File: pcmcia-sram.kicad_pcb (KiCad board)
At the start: 4 copper layers, 9 parts, among them J1 PCMCIA, U1 AS6C8008-55ZIN

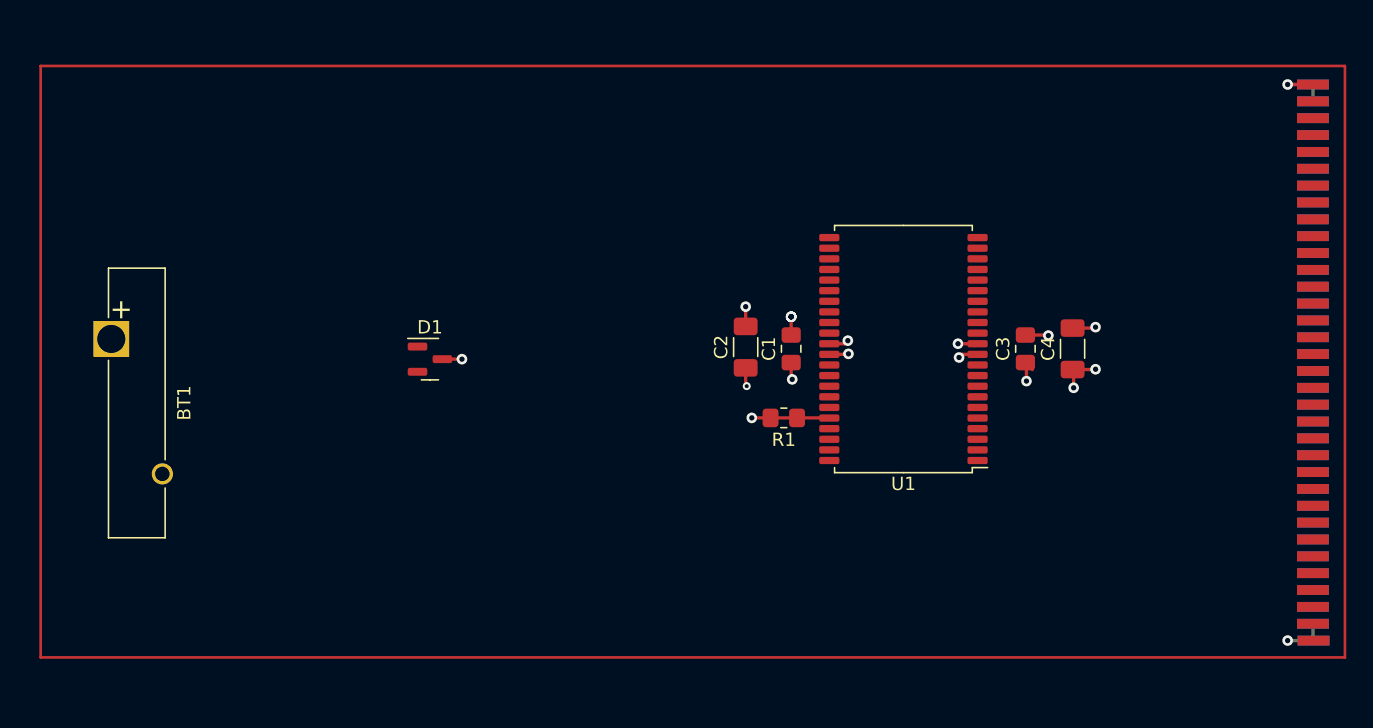
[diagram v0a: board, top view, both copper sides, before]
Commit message: Various fixes
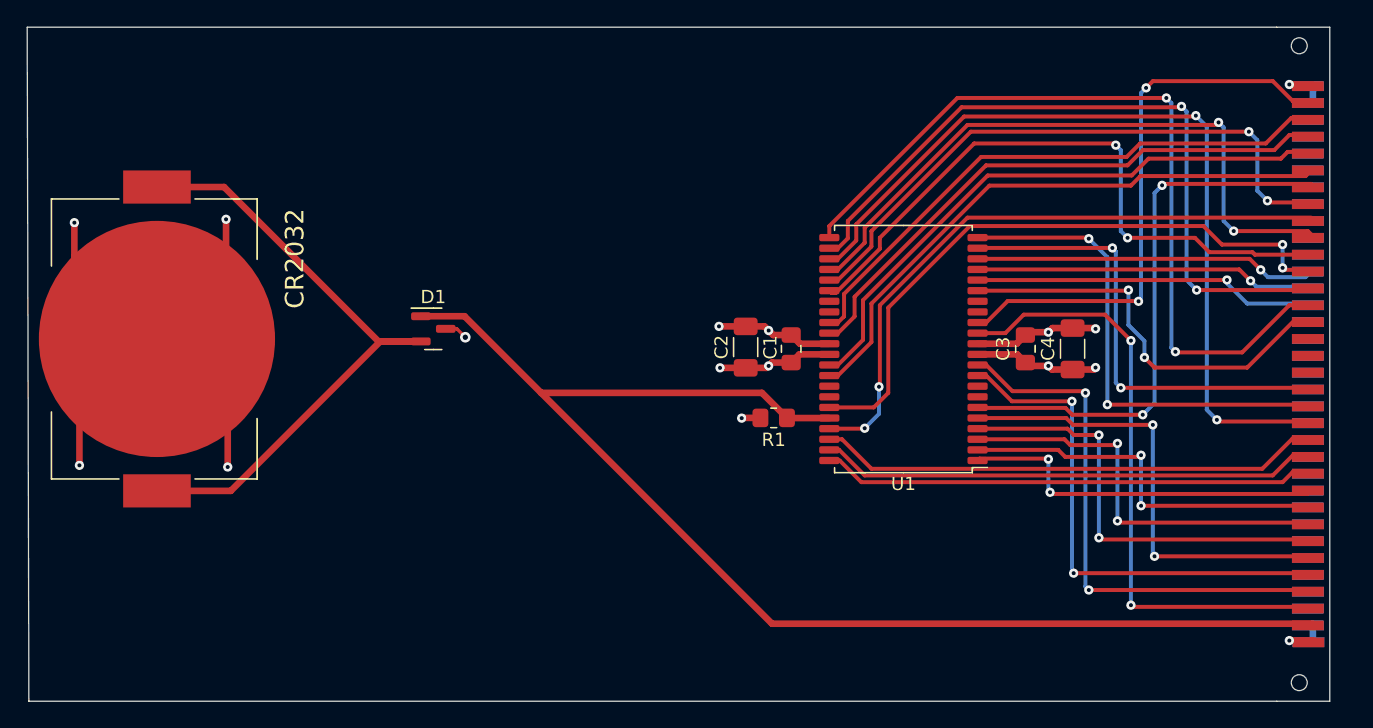
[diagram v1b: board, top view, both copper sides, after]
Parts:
- CR2032: renamed from BT1; footprint Battery:Battery_Panasonic_CR2032-VS1N_Vertical_CircularHoles -> pcmcia:BAT_BAT-HLD-001
- moved CR2032 3.44 mm to (165.5, 86.2)
- moved D1 2.30 mm to (186.3, 85.5)
- moved J1 0.76 mm to (253.9, 88.1)
- moved R1 0.76 mm to (212.0, 92.2)
- turned C1 to -90 degrees
- turned C2 to -90 degrees
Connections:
- J1 pad 64: (no net) -> unconnected-(J1-Pad64)
- U1 pad 39: /A -> /A8
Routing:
- net +5V: track 4.93 -> 99.3 mm
- net /A12: track 0.00 -> 63.7 mm, vias 0 -> 2
- net /A14: track 0.00 -> 61.2 mm, vias 0 -> 2
- net GND: track 19.0 -> 75.2 mm
- net /A13: track 0.00 -> 54.6 mm, vias 0 -> 2
- net /A11: track 0.00 -> 49.4 mm, vias 0 -> 2
- net +BATT: track 0.00 -> 49.3 mm
- net /A9: track 0.00 -> 48.3 mm, vias 0 -> 2
- net /A8: track 0.00 -> 48.3 mm, vias 0 -> 2
- net /OE: track 0.00 -> 47.6 mm, vias 0 -> 2
- net /D2: track 0.00 -> 46.7 mm, vias 0 -> 2
- net /A10: track 0.00 -> 46.2 mm, vias 0 -> 2
- net /D6: track 0.00 -> 44.9 mm
- net /D7: track 0.00 -> 44.6 mm
- net /D4: track 0.00 -> 43.8 mm
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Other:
- board outline added: 94.2 x 50.8 mm
